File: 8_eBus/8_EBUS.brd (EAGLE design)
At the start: 67.4 x 44.8 mm, 20 parts, among them IC1 MCP6542, Q1 BC817, X1 AKL18X-02W, X2 ALLSERIALSLAVE

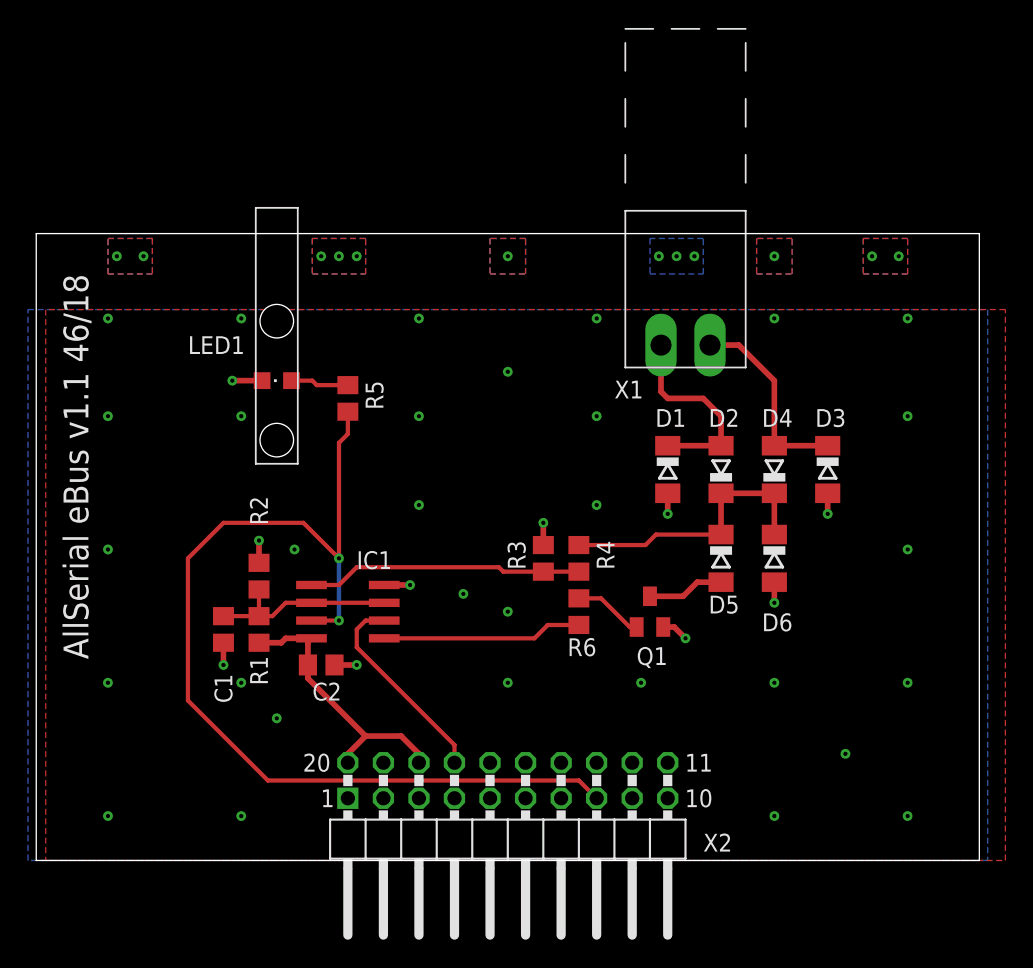
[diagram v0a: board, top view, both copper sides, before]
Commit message: Cleanup, front with lib elements
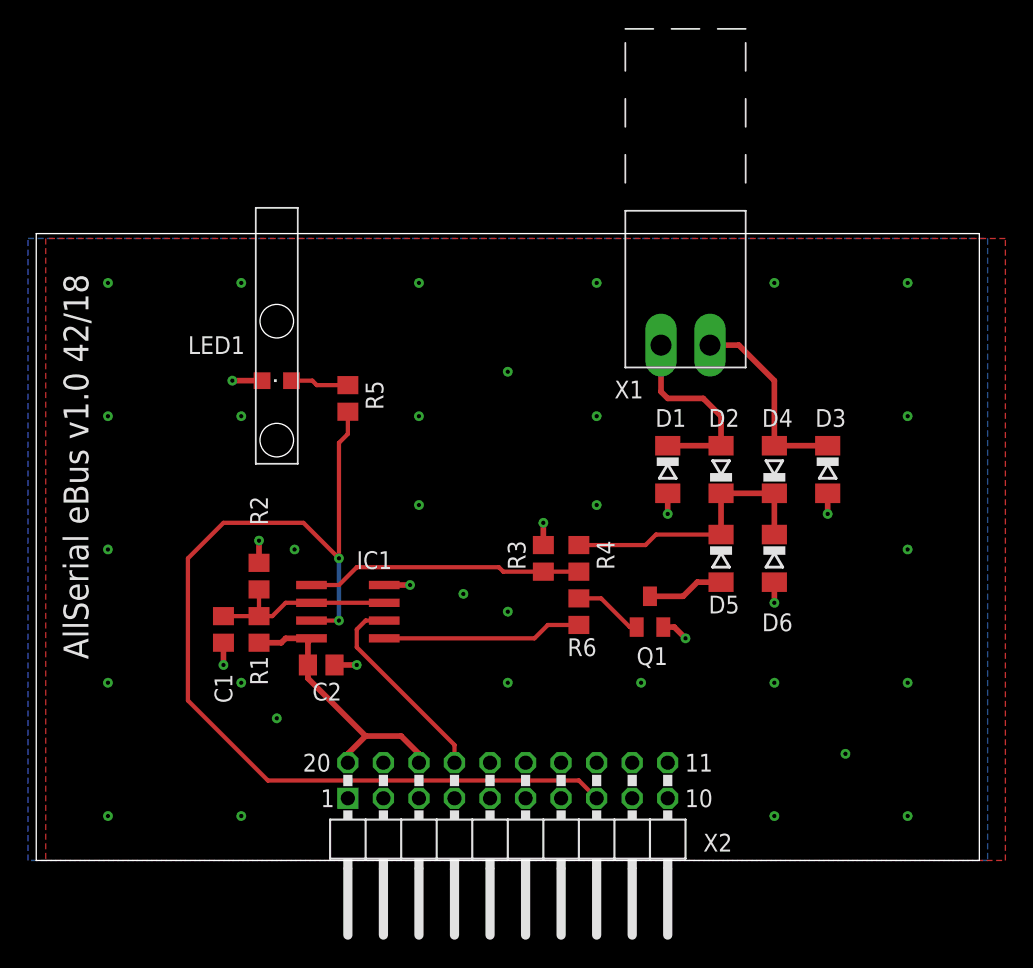
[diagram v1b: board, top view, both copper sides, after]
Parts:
- R5: value 270 -> 180
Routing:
- removed copper zone on layer 1, net N$13
- removed copper zone on layer 16, net N$13
- removed copper zone on layer 1, net N$14
- removed copper zone on layer 16, net N$14
- removed copper zone on layer 1, net N$15
- removed copper zone on layer 16, net N$15
- removed copper zone on layer 16, net N$16
- removed copper zone on layer 1, net N$17
- removed copper zone on layer 16, net N$17
- removed copper zone on layer 1, net N$6
- removed copper zone on layer 16, net N$6
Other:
- board text added: "AllSerial eBus v1.0 42/18"
- board text removed: "AllSerial eBus v1.1 46/18"
